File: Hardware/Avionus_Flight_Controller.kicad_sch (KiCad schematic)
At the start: 0 parts

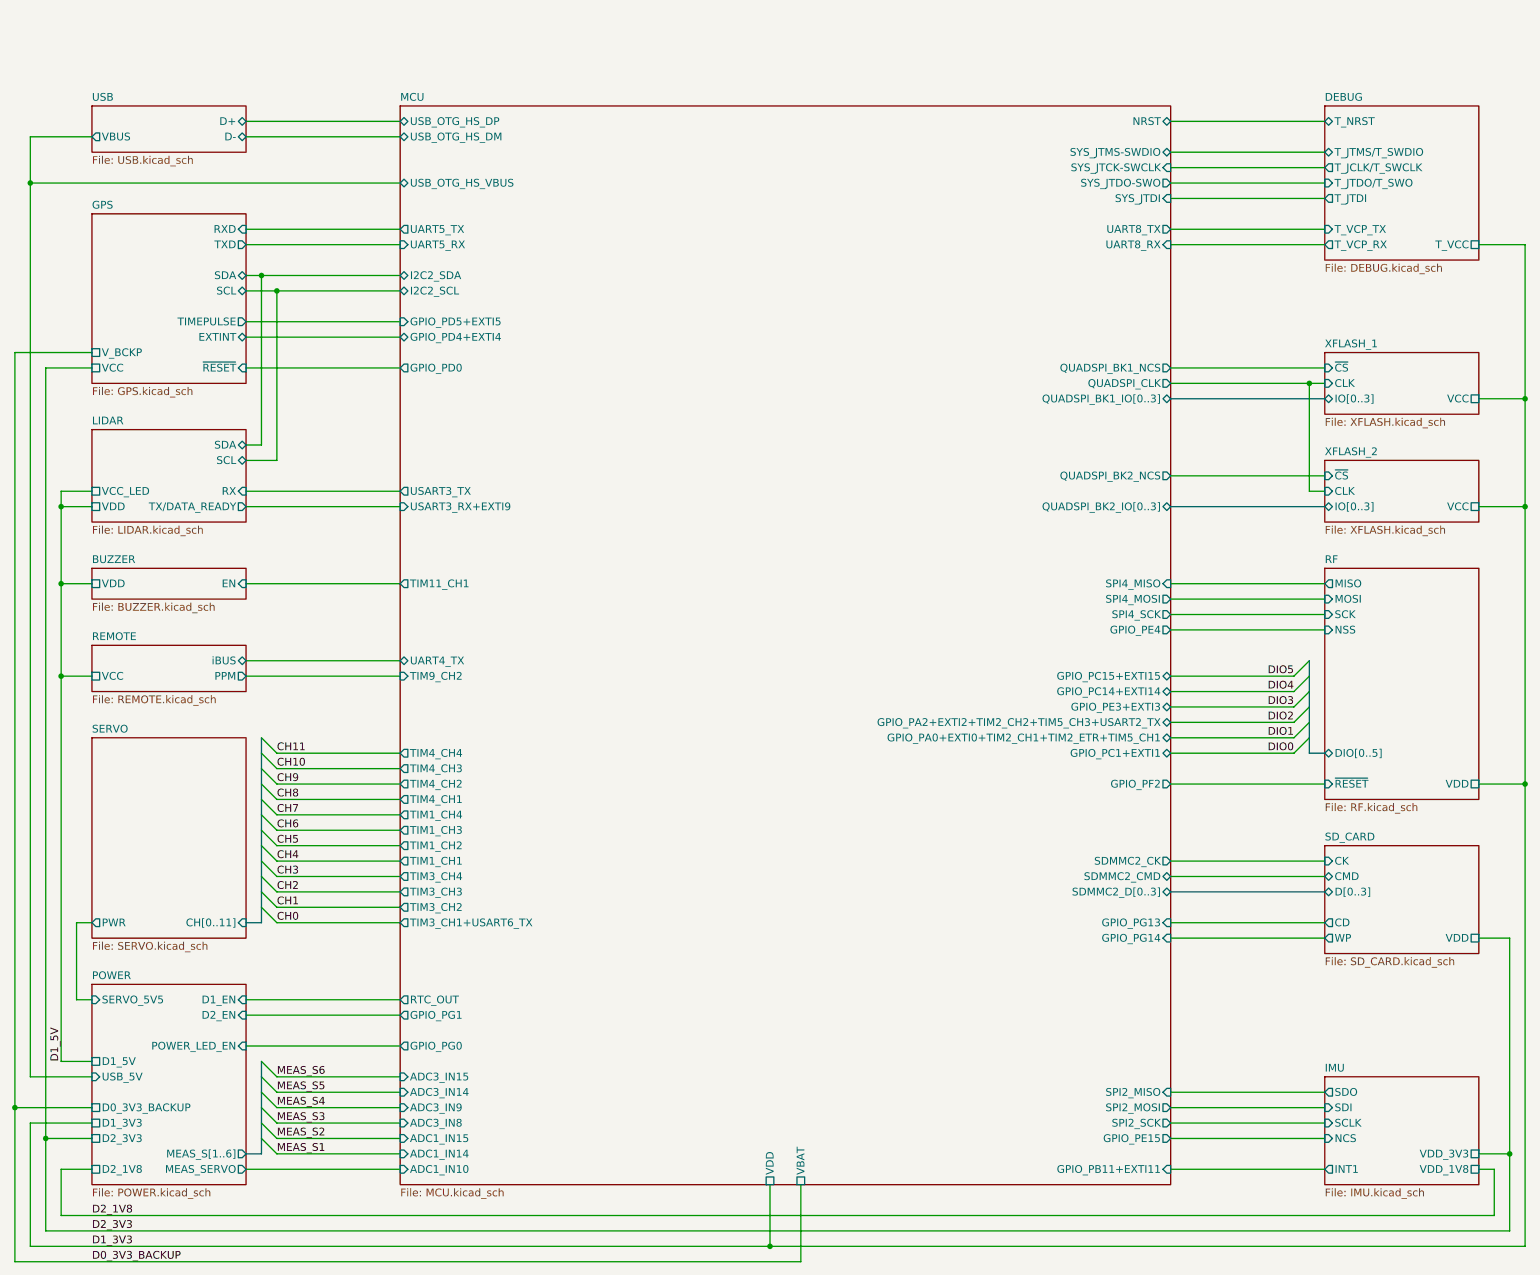
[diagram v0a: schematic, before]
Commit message: Checkpoint
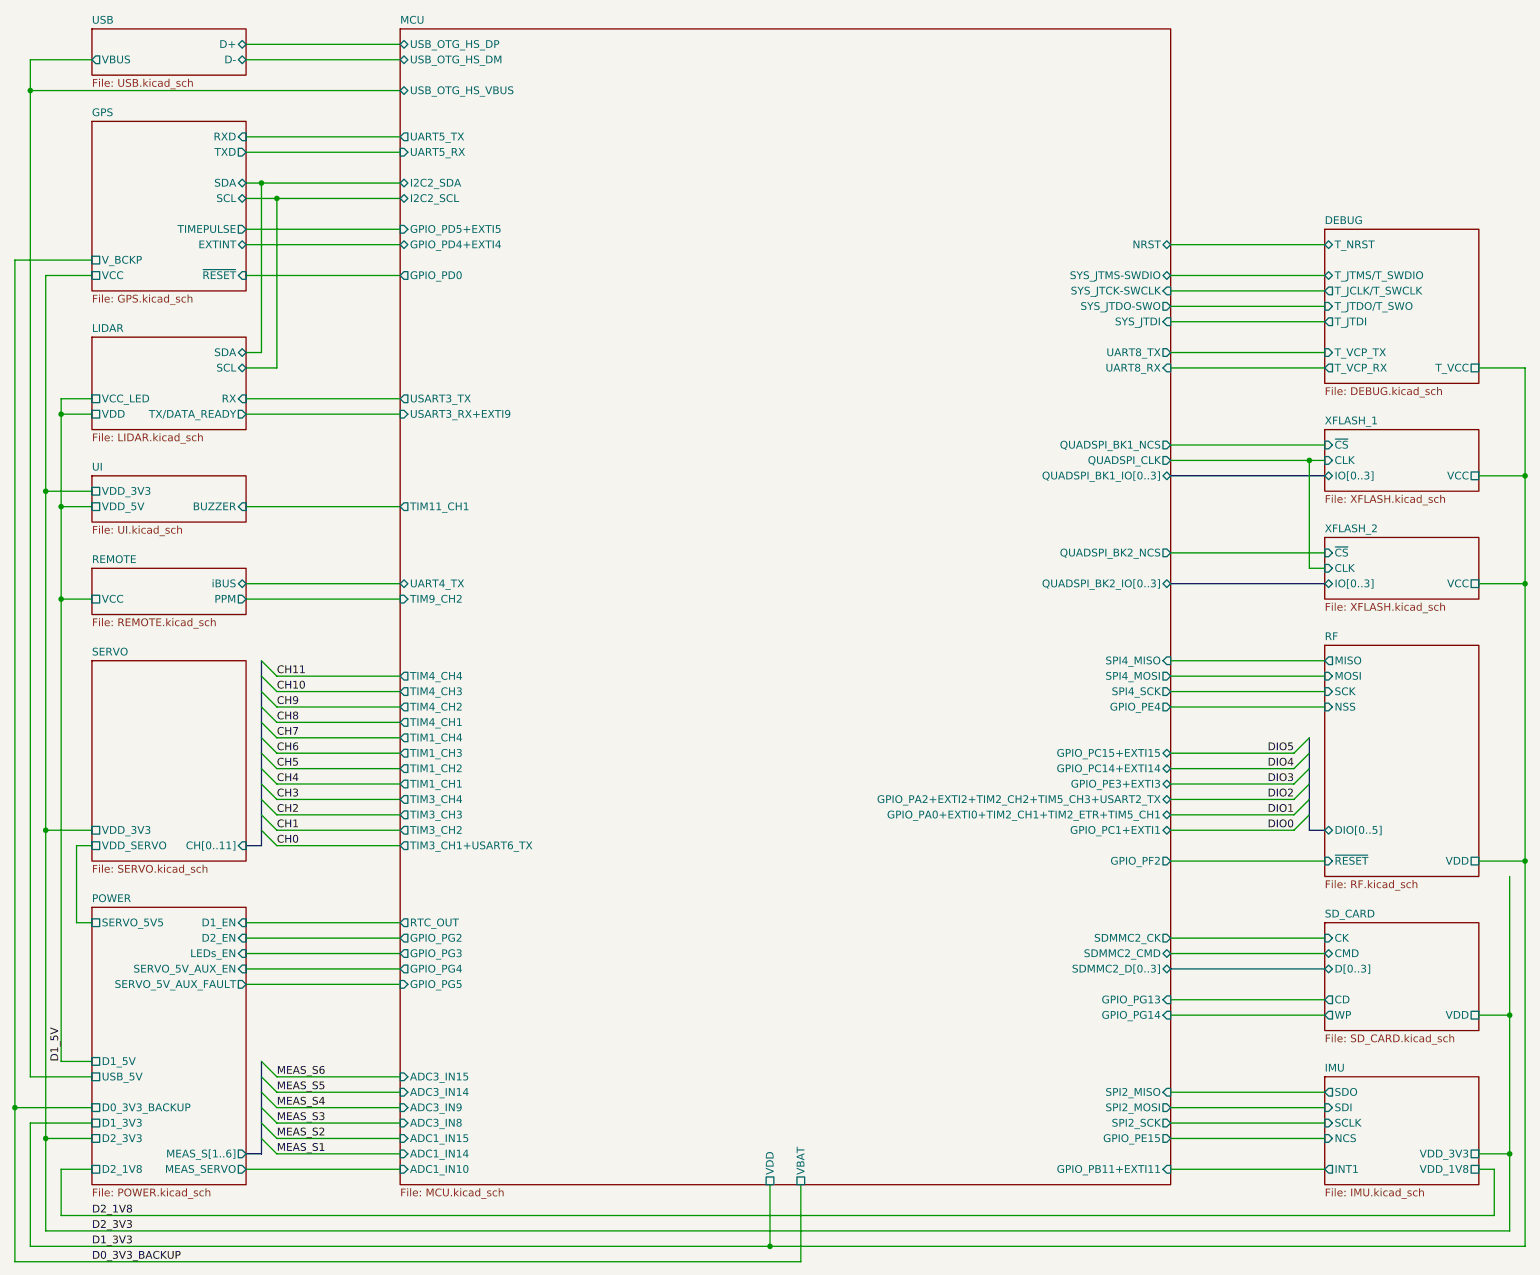
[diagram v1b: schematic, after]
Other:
- sheet BUZZER renamed UI
- sheet MCU ports: added GPIO_PG2, GPIO_PG3, GPIO_PG4, GPIO_PG5; removed GPIO_PG0, GPIO_PG1
- sheet POWER ports: added LEDs_EN, SERVO_5V_AUX_EN, SERVO_5V_AUX_FAULT; removed POWER_LED_EN
- sheet SERVO ports: added VDD_3V3, VDD_SERVO; removed PWR
- sheet UI: file BUZZER.kicad_sch -> UI.kicad_sch
- sheet UI ports: added BUZZER, VDD_3V3, VDD_5V; removed EN, VDD
